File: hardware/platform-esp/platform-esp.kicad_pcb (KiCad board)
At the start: 2 copper layers, 86 x 50.9 mm, 57 parts, among them J1 Conn_ARM_JTAG_SWD_10, J2 DM3AT-SF-PEJM5, J3 DEBUG, J4 USB_C_Receptacle_USB2.0, SW1 SW_Push, SW2 SW_Push, U1 W25Q128JVS, U2 ESP-PSRAM32, U3 ESP32-S3R2, Y1 40MHZ, Y2 32.7k

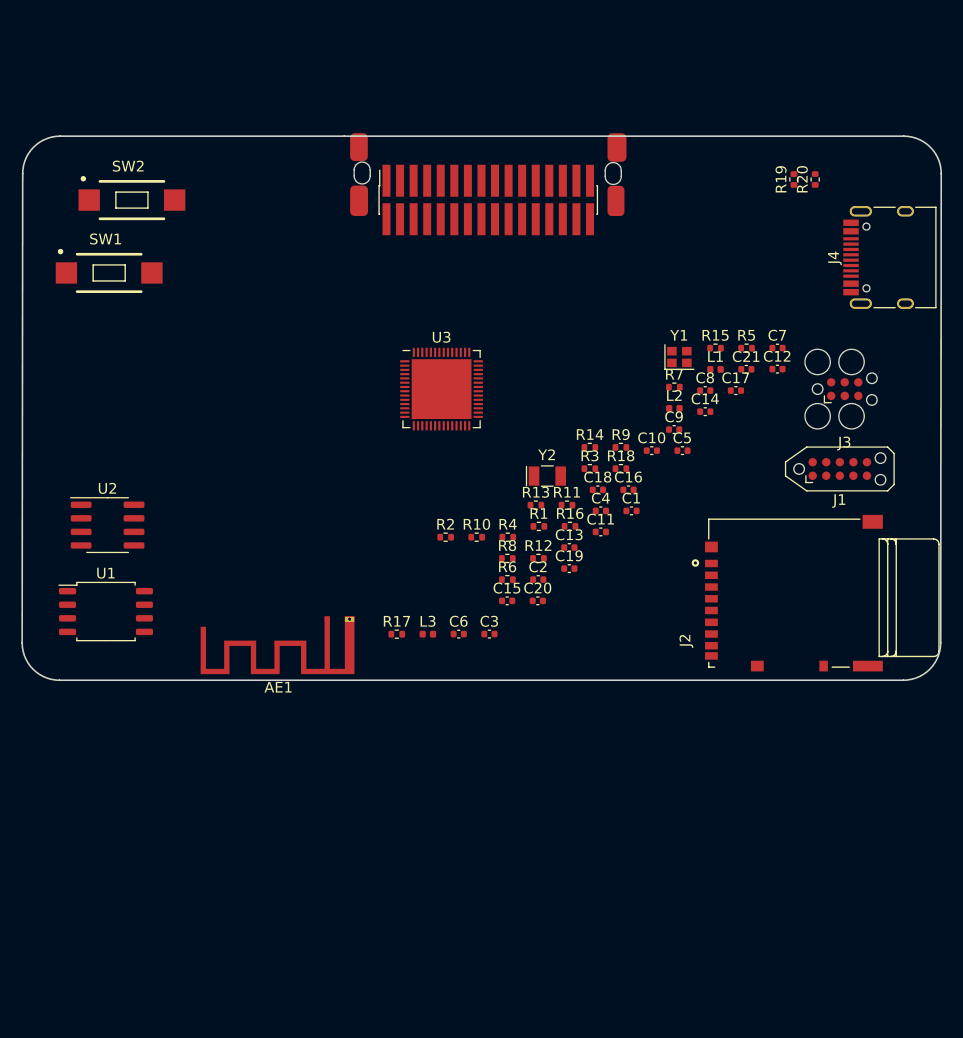
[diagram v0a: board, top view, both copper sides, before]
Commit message: circle pcb go brrrr lmao
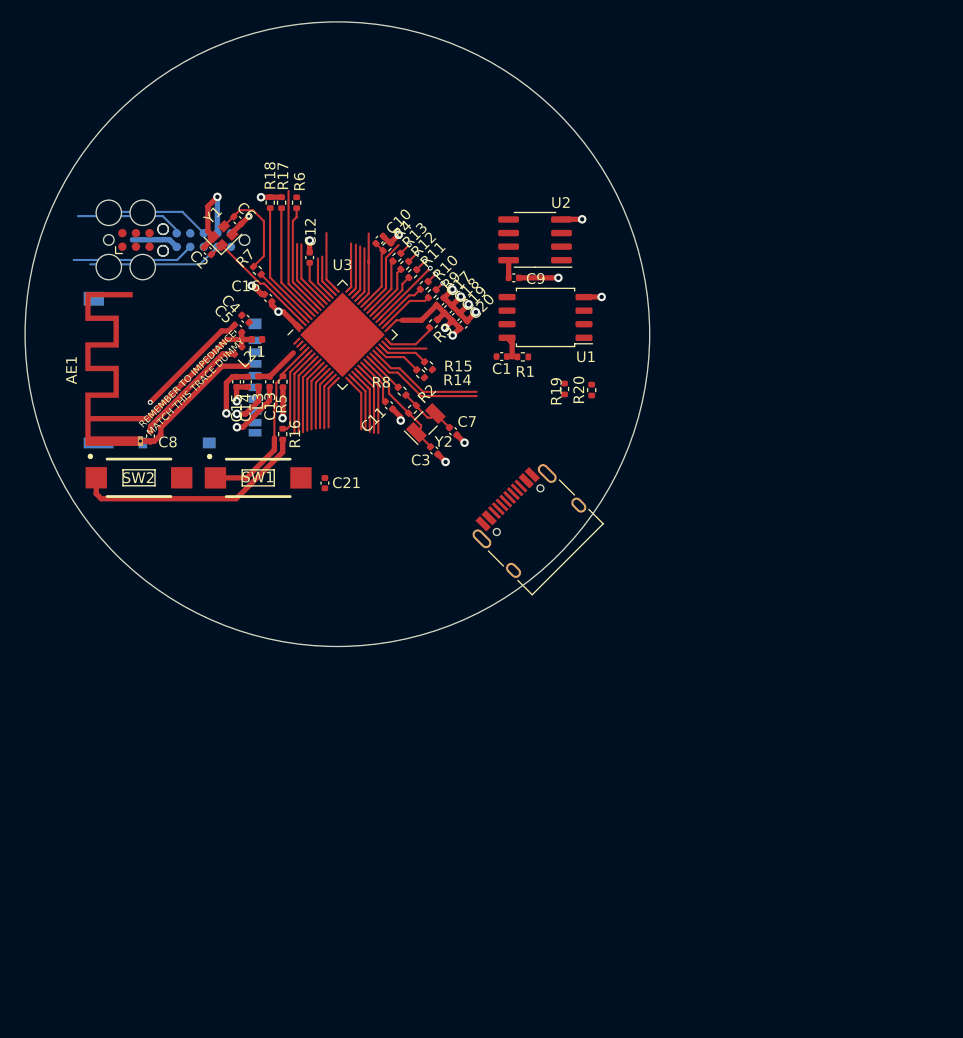
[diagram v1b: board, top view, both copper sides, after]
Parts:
- removed CONN: Conn_02x15_Odd_Even_Shielded, TE_DTM1312PA12PBR008:PinSocket_2x16_P1.27mm_Vertical_SMD
- J1, J2: moved to B.Cu
- moved J3 67.8 mm to (25.5, 24.7)
- moved J1 63.3 mm to (31.8, 24.7), turned to 180 degrees
- moved C8 52.1 mm to (26.8, 43.0), turned to 90 degrees
- moved U1 49.5 mm to (63.8, 31.9), turned to 180 degrees
- moved U2 48.1 mm to (62.8, 24.7), turned to 180 degrees
- moved J2 47.5 mm to (36.6, 37.3)
- moved C12 45.0 mm to (41.7, 26.3), turned to 90 degrees
- moved Y1 44.2 mm to (33.6, 24.3), turned to 45 degrees
- moved C6 43.9 mm to (35.0, 22.8), turned to -45 degrees
- moved C2 43.6 mm to (32.2, 25.7), turned to 135 degrees
- moved R5 43.5 mm to (39.2, 38.0), turned to -90 degrees
- moved C5 43.1 mm to (35.0, 33.0), turned to -45 degrees
- moved L1 43.0 mm to (36.8, 34.0), turned to 180 degrees
- moved C14 42.9 mm to (35.9, 38.0), turned to -90 degrees
- moved J4 42.0 mm to (63.1, 51.8), turned to 45 degrees
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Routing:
- net GND: track 0.00 -> 74.8 mm, vias 0 -> 19
- net +3V3: track 0.00 -> 31.6 mm, vias 0 -> 6
- net /GPIO0_BOOTSTRAP: track 0.00 -> 22.1 mm
- net /MTMS: track 0.00 -> 19.2 mm
- net /CHIP_PU: track 0.00 -> 17.2 mm
- net /MTDI: track 0.00 -> 16.2 mm
- net /MTCK: track 0.00 -> 15.2 mm
- net Net-(AE1-Pad1): track 0.00 -> 14.8 mm
- net /MTDO: track 0.00 -> 14.0 mm
- net /U0RXD: track 0.00 -> 12.2 mm
- net /XTAL_P: track 0.00 -> 11.9 mm
- net /GPIO46: track 0.00 -> 11.7 mm
- net /GPIO17: track 0.00 -> 11.2 mm
- net Net-(C8-Pad2): track 0.00 -> 11.1 mm
- net /GPIO45: track 0.00 -> 11.0 mm
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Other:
- board size 86 x 50.9 mm -> 58.5 x 58.5 mm
- copper layers 2 -> 4
- board text added: "REMEMBER TO IMPEDIANCE MATCH THIS TRACE DUMMY"

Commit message: backup
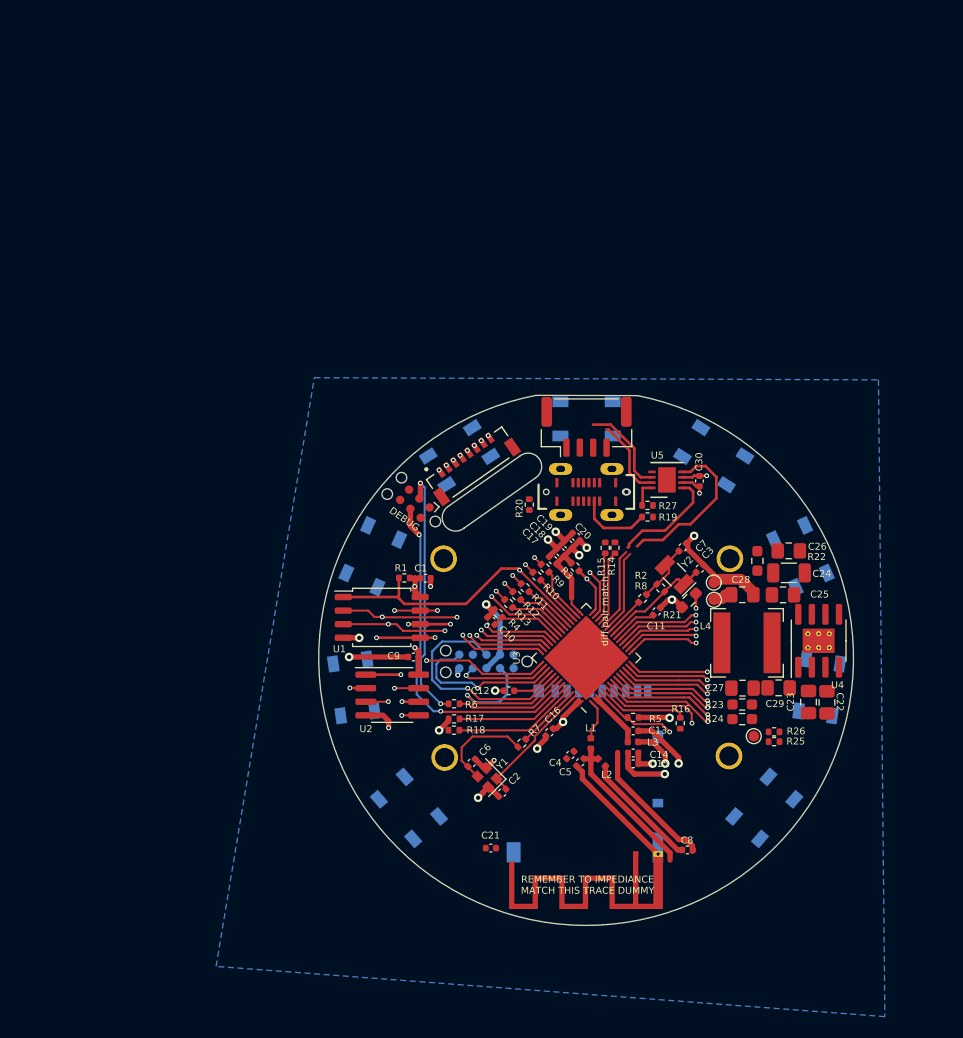
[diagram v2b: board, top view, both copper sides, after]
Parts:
- removed SW1, SW2: SW_Push, SW_RS-032G05A3-SMRT:SW_RS-032G05A3-SMRT
- added C22: 10uf, Capacitor_SMD:C_0805_2012Metric_Pad1.18x1.45mm_HandSolder, F.Cu at (90.2, 68.0)
- added C23: 10uf, Capacitor_SMD:C_0805_2012Metric_Pad1.18x1.45mm_HandSolder, F.Cu at (88.4, 67.9)
- added C24: 5.6nf, Capacitor_SMD:C_1206_3216Metric, F.Cu at (86.6, 55.9)
- added C25: 0.1uf, Capacitor_SMD:C_0805_2012Metric_Pad1.18x1.45mm_HandSolder, F.Cu at (86.0, 57.9)
- added C26: DNP, Capacitor_SMD:C_0805_2012Metric_Pad1.18x1.45mm_HandSolder, F.Cu at (86.6, 53.8)
- added C27: DNP, Capacitor_SMD:C_0805_2012Metric_Pad1.18x1.45mm_HandSolder, F.Cu at (82.2, 66.6)
- added C28: DNP, Capacitor_SMD:C_0805_2012Metric_Pad1.18x1.45mm_HandSolder, F.Cu at (82.2, 57.9)
- added C29: DNP, Capacitor_SMD:C_0805_2012Metric_Pad1.18x1.45mm_HandSolder, F.Cu at (85.6, 66.6)
- added C30: 0.1uF, Capacitor_SMD:C_0402_1005Metric, F.Cu at (78.2, 47.3)
- added D1: WS2812B, LED_SMD:LED_WS2812B_PLCC4_5.0x5.0mm_P3.2mm, B.Cu at (67.7, 41.4)
- added D10: WS2812B, LED_SMD:LED_WS2812B_PLCC4_5.0x5.0mm_P3.2mm, B.Cu at (47.6, 54.3)
- added D11: WS2812B, LED_SMD:LED_WS2812B_PLCC4_5.0x5.0mm_P3.2mm, B.Cu at (55.8, 44.9)
- added D2: WS2812B, LED_SMD:LED_WS2812B_PLCC4_5.0x5.0mm_P3.2mm, B.Cu at (79.5, 44.9)
- added D3: WS2812B, LED_SMD:LED_WS2812B_PLCC4_5.0x5.0mm_P3.2mm, B.Cu at (87.7, 54.3)
- added D4: WS2812B, LED_SMD:LED_WS2812B_PLCC4_5.0x5.0mm_P3.2mm, B.Cu at (89.4, 66.6)
- added D5: WS2812B, LED_SMD:LED_WS2812B_PLCC4_5.0x5.0mm_P3.2mm, B.Cu at (84.3, 77.8)
- added D8: WS2812B, LED_SMD:LED_WS2812B_PLCC4_5.0x5.0mm_P3.2mm, B.Cu at (51.0, 77.8)
- added D9: WS2812B, LED_SMD:LED_WS2812B_PLCC4_5.0x5.0mm_P3.2mm, B.Cu at (45.9, 66.6)
- added J5: DF52-8S-0.8H(21), Connector_Hirose_SD:HIROSE_DF52-8S-0.8H(21), F.Cu at (56.3, 44.8)
- added J6: TC2030-IDC, Connector:Tag-Connect_TC2030-IDC-NL_2x03_P1.27mm_Vertical, F.Cu at (51.6, 49.4)
- added L4: 6.8uh, Inductor_SMD:L_Bourns-SRN6028, F.Cu at (82.7, 62.4)
- added R21: 200k, Resistor_SMD:R_0603_1608Metric_Pad0.98x0.95mm_HandSolder, F.Cu at (77.2, 58.4)
- added R22: 14k, Resistor_SMD:R_0603_1608Metric_Pad0.98x0.95mm_HandSolder, F.Cu at (83.6, 54.7)
- added R23: 52.3k, Resistor_SMD:R_0603_1608Metric_Pad0.98x0.95mm_HandSolder, F.Cu at (82.2, 68.2)
- added R24: 10k, Resistor_SMD:R_0603_1608Metric_Pad0.98x0.95mm_HandSolder, F.Cu at (82.2, 69.5)
- added R25: 36k, Resistor_SMD:R_0402_1005Metric, F.Cu at (85.2, 71.6)
- added R26: 10k, Resistor_SMD:R_0402_1005Metric, F.Cu at (85.2, 70.7)
- added R27: 10k, Resistor_SMD:R_0402_1005Metric, F.Cu at (73.4, 49.5)
- added REF**: 1.28-lcd, Module_Waveshare:1.28-lcd, B.Cu at (67.7, 63.8)
- added TP1: 3V3OUT, TestPoint:TestPoint_Pad_D1.0mm, F.Cu at (79.6, 56.8)
- added TP2: 3V3OUT, TestPoint:TestPoint_Pad_D1.0mm, F.Cu at (79.6, 58.4)
- added TP3: VBAT_SENSE, TestPoint:TestPoint_Pad_D1.0mm, F.Cu at (83.3, 71.1)
- added U4: AP64200Q, Package_SO:SOIC-8-1EP_3.9x4.9mm_P1.27mm_EP2.29x3mm_ThermalVias, F.Cu at (89.4, 62.2)
- added U5: LTC2875-DD, Package_DFN_QFN:DFN-8-1EP_3x3mm_P0.5mm_EP1.66x2.38mm, F.Cu at (75.2, 47.1)
- J3: value DEBUG -> Conn_01x04_Male; footprint Connector:Tag-Connect_TC2030-IDC-FP_2x03_P1.27mm_Vertical -> Connector_JST:JST_GH_BM04B-GHS-TBT_1x04-1MP_P1.25mm_Vertical
- J4: value USB_C_Receptacle_USB2.0 -> USB4120-03-C_REVA; footprint Connector_USB:USB_C_Receptacle_HRO_TYPE-C-31-M-12 -> Connector_GCT_USB:GCT_USB4120-03-C_REVA
- moved C8 63.5 mm to (77.1, 81.8), turned to 180 degrees
- moved AE1 61.7 mm to (72.2, 82.2), turned to 180 degrees
- moved C2 57.7 mm to (59.8, 76.4), turned to -135 degrees
- moved Y1 56.4 mm to (58.3, 75.0), turned to 135 degrees
- moved C6 55.3 mm to (56.9, 73.6), turned to 45 degrees
- moved R18 52.3 mm to (55.2, 70.6), turned to 180 degrees
- moved C5 51.7 mm to (67.1, 73.6), turned to 45 degrees
- moved C15 51.5 mm to (72.0, 73.7), turned to 0 degrees
- moved L2 51.5 mm to (69.1, 73.6), turned to -45 degrees
- moved R17 50.9 mm to (55.3, 69.5), turned to 180 degrees
- moved C4 50.9 mm to (66.1, 72.9), turned to 45 degrees
- moved R7 50.7 mm to (61.6, 71.8), turned to 45 degrees
- moved C14 50.1 mm to (72.0, 72.7), turned to 0 degrees
- moved R6 49.2 mm to (55.3, 68.1), turned to 0 degrees
- moved L1 49.1 mm to (68.0, 71.8), turned to -90 degrees
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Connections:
- J4 pad A1: Net-(J4-PadA1) -> GND
- J4 pad A12: Net-(J4-PadA1) -> GND
- J4 pad A4: Net-(J4-PadA4) -> unconnected-(J4-PadA4)
- J4 pad A5: unconnected-(J4-PadA5) -> /CC1
- J4 pad A9: Net-(J4-PadA4) -> unconnected-(J4-PadA4)
- J4 pad B1: Net-(J4-PadA1) -> GND
- J4 pad B12: Net-(J4-PadA1) -> GND
- J4 pad B4: Net-(J4-PadA4) -> unconnected-(J4-PadB4)
- J4 pad B5: unconnected-(J4-PadB5) -> /CC2
- J4 pad B9: Net-(J4-PadA4) -> unconnected-(J4-PadB4)
- J4 pad S1: unconnected-(J4-PadS1) -> Net-(J4-PadS1)
- R19 pad 1: unconnected-(R19-Pad1) -> /CC2
- R19 pad 2: unconnected-(R19-Pad2) -> GND
- R20 pad 1: unconnected-(R20-Pad1) -> /CC1
- R20 pad 2: unconnected-(R20-Pad2) -> GND
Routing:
- net /SPIWP: track 1.01 -> 32.1 mm, vias 1 -> 4
- net /SPIQ: track 1.09 -> 30.8 mm, vias 1 -> 4
- net /SPICS1: track 4.80 -> 34.0 mm, vias 0 -> 2
- net /SPIHD: track 0.89 -> 26.2 mm, vias 1 -> 4
- net /U0TXD: track 0.00 -> 24.0 mm, vias 0 -> 2
- net /SPID: track 1.26 -> 23.9 mm, vias 1 -> 4
- net /GPIO0_BOOTSTRAP: track 22.1 -> 0.00 mm
- net /SPICLK: track 1.12 -> 23.2 mm, vias 1 -> 4
- net /U0RXD: track 12.2 -> 33.2 mm, vias 0 -> 2
- net /SPICS0: track 6.79 -> 26.9 mm
- net /CAN_N: track 0.00 -> 15.2 mm
- net /CAN_P: track 0.00 -> 10.2 mm
- net /CHIP_PU: track 17.2 -> 7.83 mm, vias 0 -> 1
- net /CAN_DRV_N: track 0.00 -> 8.80 mm
- net /CAN_DRV_P: track 0.00 -> 7.56 mm
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- added copper zone on In2.Cu, net +3V3
- added copper zone on B.Cu, net GND
- added copper zone on In1.Cu, net GND
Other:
- board size 58.5 x 58.5 mm -> 50 x 49.6 mm
- board text added: "DEBUG"
- board text added: "diff pair match"
